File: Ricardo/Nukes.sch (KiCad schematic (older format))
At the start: 21 parts, among them J6 Screw_Terminal_01x02, J7 Screw_Terminal_01x02, J8 Screw_Terminal_01x02, Q4 PMV20ENR, Q5 PMV20ENR, U10 LTV-817S, U9 LTV-817S

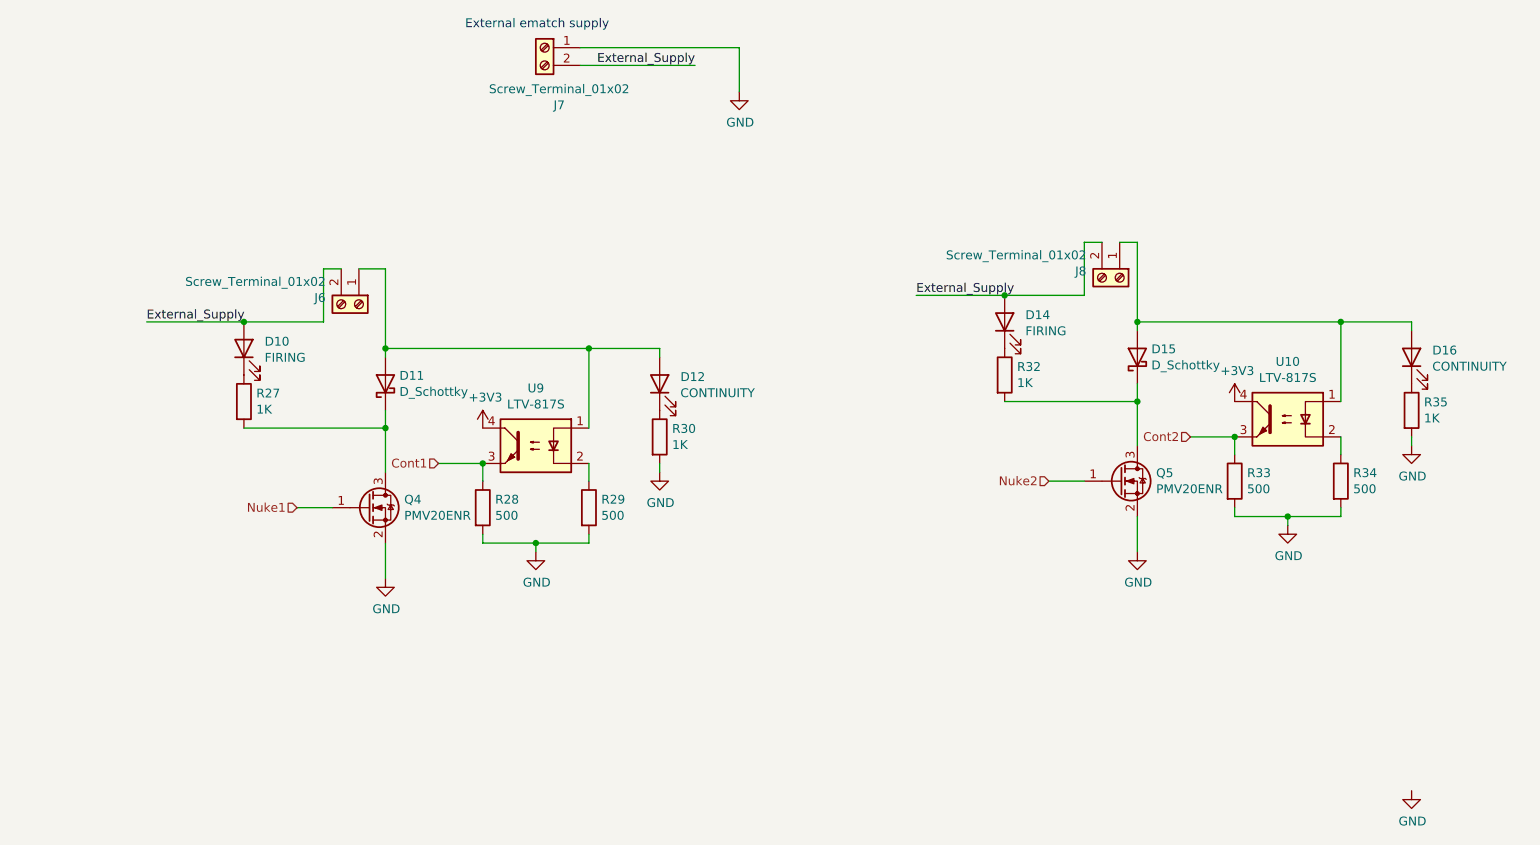
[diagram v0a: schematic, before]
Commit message: SANIC Branch
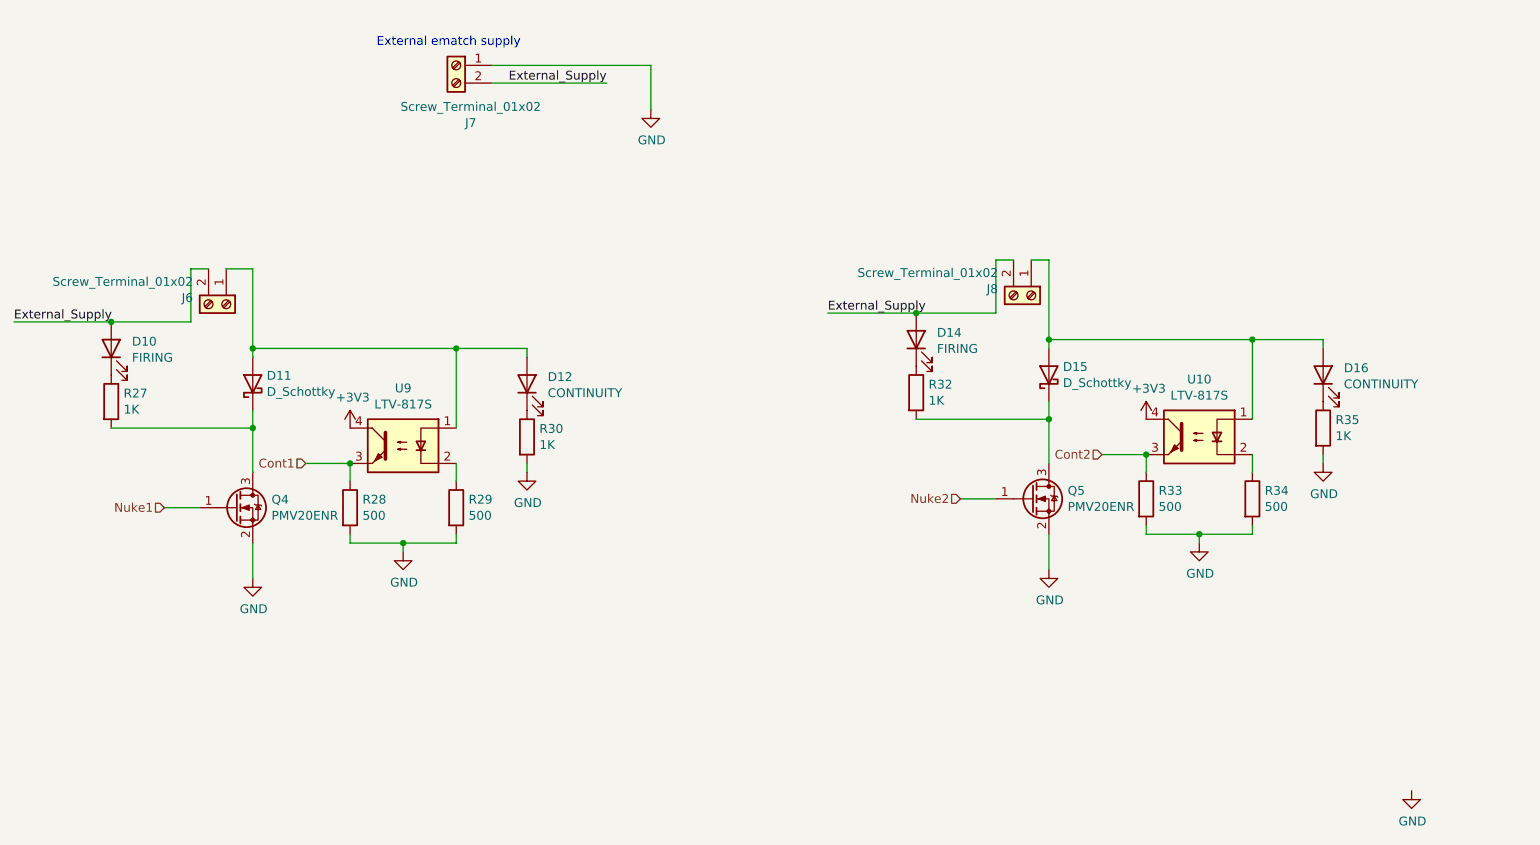
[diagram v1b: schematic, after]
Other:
- moved on the sheet: D10, D11, D12, D14, D15, D16, J6, J7, J8, Q4, Q5, R27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
